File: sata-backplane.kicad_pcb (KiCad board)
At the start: 4 copper layers, 50 x 50 mm, 10 parts, among them J1 SATA_POWER_15, J10 SATA_1, J11 SATA_COMBINED_1, J20 SATA_2, J21 SATA_COMBINED_2

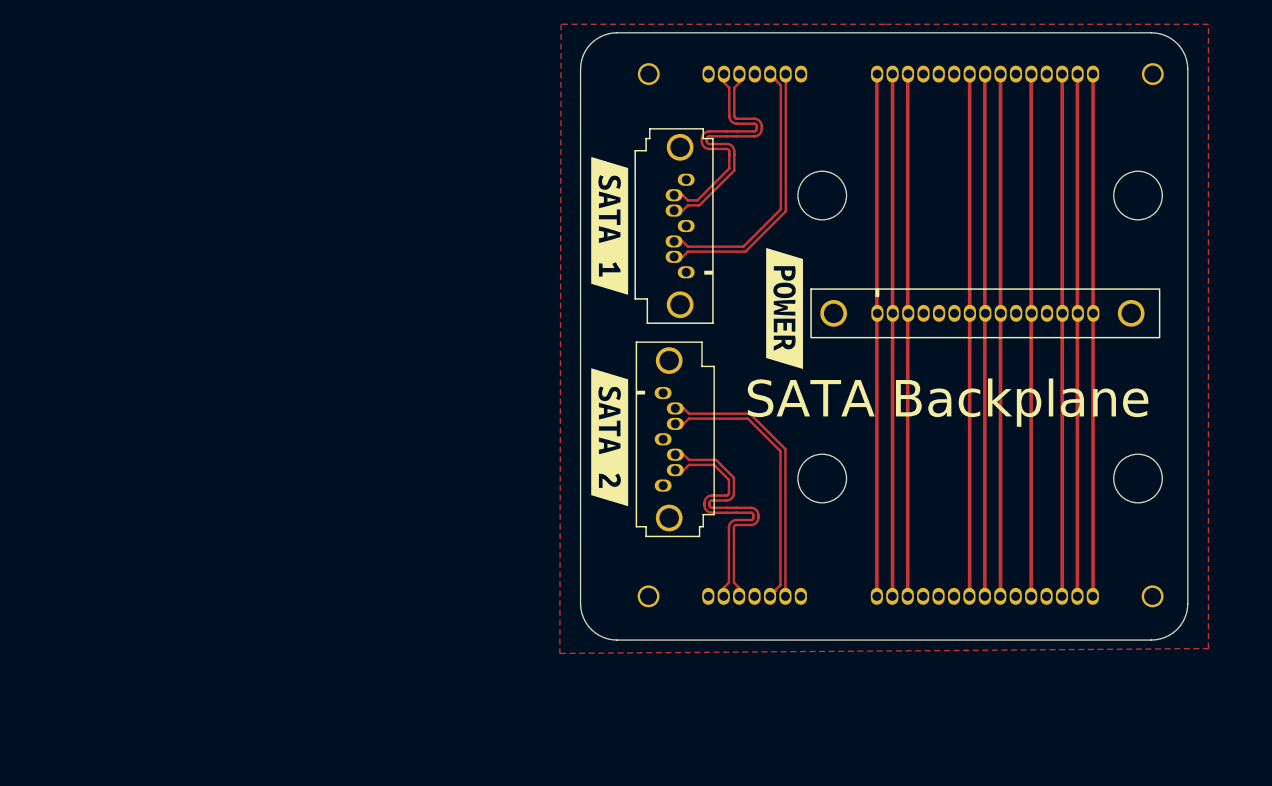
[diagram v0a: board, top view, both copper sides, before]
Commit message: Done, New parts & spacing
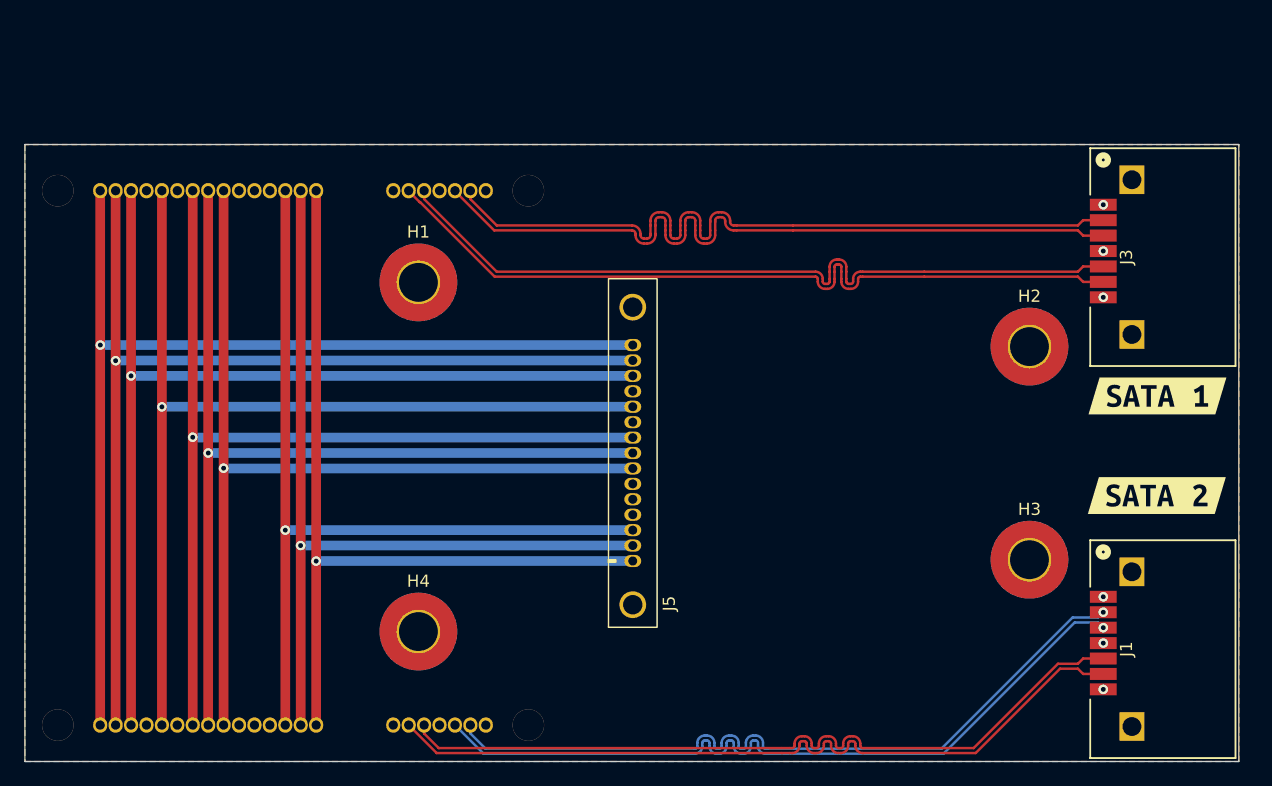
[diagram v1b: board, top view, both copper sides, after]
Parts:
- removed J10: SATA_1, sata:SATA_Data
- removed J11: SATA_COMBINED_1, sata:SATA_Combined
- removed J20: SATA_2, sata:SATA_Data
- removed J21: SATA_COMBINED_2, sata:SATA_Combined
- removed kibuzzard-63B1B180: G***, kibuzzard-63B1B180
- added H1: MountingHole_Pad, MountingHole:MountingHole_3.2mm_M3_Pad_TopBottom, F.Cu at (66.8, 45.1)
- added H2: MountingHole_Pad, MountingHole:MountingHole_3.2mm_M3_Pad_TopBottom, F.Cu at (117.1, 50.4)
- added H3: MountingHole_Pad, MountingHole:MountingHole_3.2mm_M3_Pad_TopBottom, F.Cu at (117.1, 68.0)
- added H4: MountingHole_Pad, MountingHole:MountingHole_3.2mm_M3_Pad_TopBottom, F.Cu at (66.8, 73.9)
- added J2: 877791001, CONN_877791001_MOL:CONN_877791001_MOL, B.Cu at (72.3, 81.6)
- added J3: 470804001, CONN_47080-4001_MOL:CONN_47080-4001_MOL, F.Cu at (128.0, 43.1)
- added J4: 877791001, CONN_877791001_MOL:CONN_877791001_MOL, B.Cu at (72.3, 37.6)
- added J5: SATA_POWER_15, sata:SATA_Power, F.Cu at (84.4, 68.1)
- J1: value SATA_POWER_15 -> 470804001; footprint sata:SATA_Power -> CONN_47080-4001_MOL:CONN_47080-4001_MOL
- moved kibuzzard-63B1B17B 51.0 mm to (56.2, 76.5)
- moved kibuzzard-63B1B175 50.5 mm to (56.2, 42.5)
- moved kibuzzard-63B1B175 47.2 mm to (127.6, 54.5), turned to 0 degrees
- moved kibuzzard-63B1B17B 45.3 mm to (127.5, 62.7), turned to 0 degrees
- moved J1 36.3 mm to (128.0, 75.3), turned to 90 degrees
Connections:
- J1 pad 1: /3V3_1 -> GND
- J1 pad 2: /3V3_2 -> /SATA1_A+
- J1 pad 3: /PWDIS -> /SATA1_A-
- J1 pad 5: GND -> /SATA1_B+
- J1 pad 6: GND -> /SATA1_B-
- J1 pad 7: /5V_1 -> GND
- J1 pad 8: /5V_2 -> (no net)
- J1 pad 9: /5V_3 -> (no net)
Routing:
- net /12V_B: track 0.00 -> 87.8 mm, vias 0 -> 1
- net /12V_A: track 0.00 -> 86.6 mm, vias 0 -> 1
- net /12V_PRE: track 0.00 -> 85.3 mm, vias 0 -> 1
- net /SS/ACT: track 0.00 -> 82.8 mm, vias 0 -> 1
- net /5V_B: track 0.00 -> 80.2 mm, vias 0 -> 1
- net /5V_A: track 0.00 -> 78.9 mm, vias 0 -> 1
- net /5V_PRE: track 0.00 -> 77.7 mm, vias 0 -> 1
- net /PW_DIS: track 0.00 -> 72.6 mm, vias 0 -> 1
- net /3V3_B: track 0.00 -> 71.3 mm, vias 0 -> 1
- net /3V3_A: track 0.00 -> 70.1 mm, vias 0 -> 1
- net /SATA1_B-: track 21.7 -> 64.8 mm
- net /5V_3: track 43.0 -> 0.00 mm
- net /3V3_2: track 43.0 -> 0.00 mm
- net /12V_1: track 43.0 -> 0.00 mm
- net /PWDIS: track 43.0 -> 0.00 mm
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- added copper zone on B.Cu, net GND
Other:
- board size 50 x 50 mm -> 100 x 50.8 mm
- board text removed: "SATA Backplane"
